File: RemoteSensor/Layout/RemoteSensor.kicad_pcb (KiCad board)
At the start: 2 copper layers, 50.8 x 50.8 mm, 47 parts, among them J1 PRG_HEADER, J2 LCD_HEADER, J3 USB_B_Micro, J4 BATT_CONN, Q1 2N7002, Q2 2N7002, Q3 2N7002, SW1 BTN_RST, SW2 BTN_LOAD, SW3 SW_DPDT_x2, U1 ESP-12F, U2 74LVC2G02, U3 LM50CIM3, U4 MCP73831-2-OT, U5 LM3670MF, U6 BD48ExxG, U7 BD48ExxG

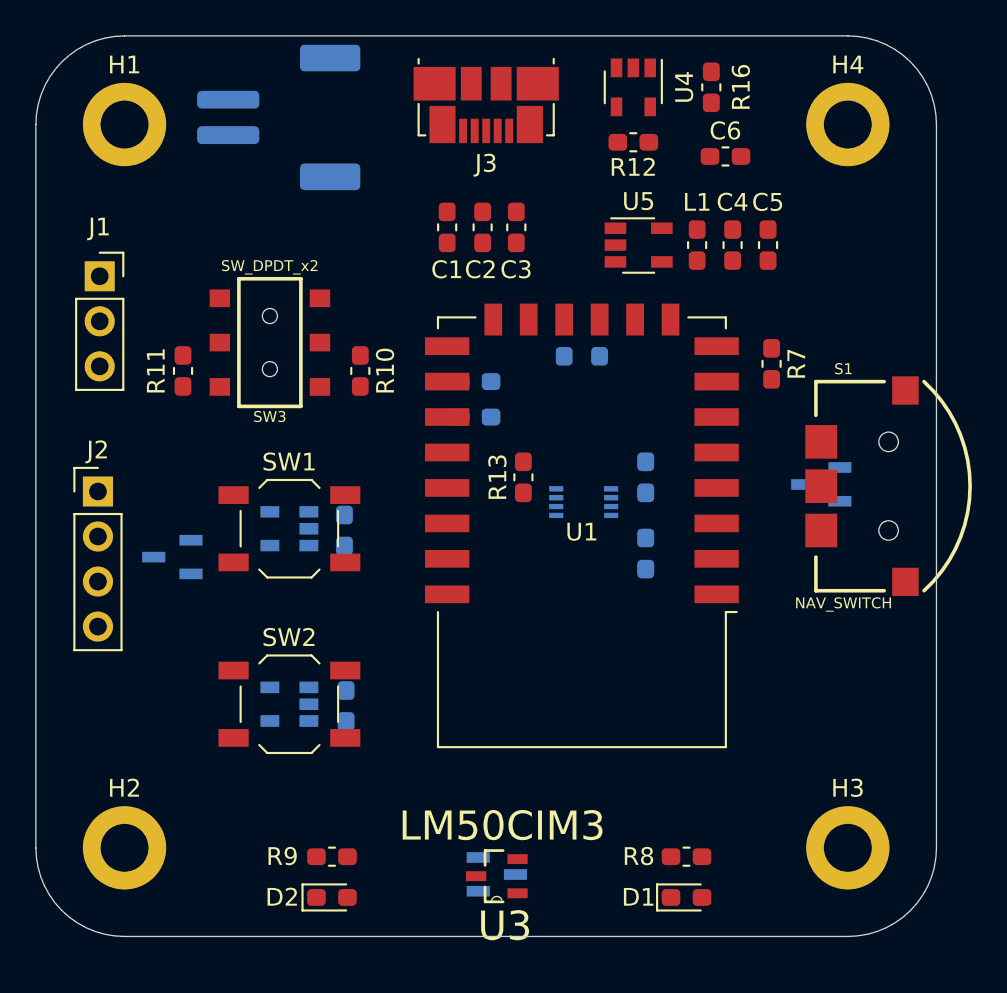
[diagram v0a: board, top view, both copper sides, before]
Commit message: Autotrace
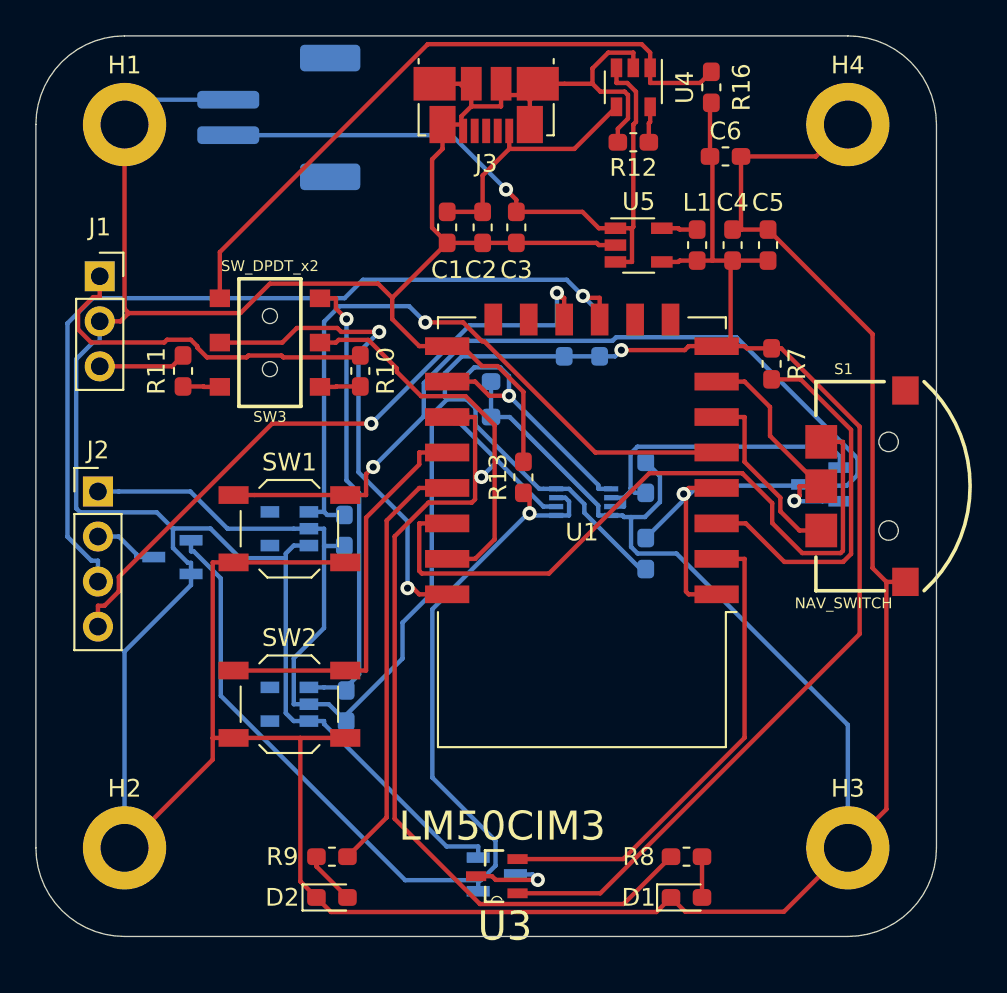
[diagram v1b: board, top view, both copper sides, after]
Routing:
- net GND: track 0.00 -> 335.7 mm
- net 3.3V: track 0.00 -> 149.5 mm, vias 0 -> 1
- net /RST: track 0.00 -> 67.6 mm, vias 0 -> 2
- net /WAKE_STS: track 0.00 -> 59.2 mm, vias 0 -> 1
- net /HB_PIN: track 0.00 -> 55.6 mm, vias 0 -> 1
- net /SCL: track 0.00 -> 50.2 mm, vias 0 -> 1
- net /UP_PIN: track 0.00 -> 40.5 mm
- net /BATT_STS: track 0.00 -> 38.7 mm, vias 0 -> 1
- net V_BATT: track 0.00 -> 38.1 mm, vias 0 -> 1
- net /SDA: track 0.00 -> 38.1 mm, vias 0 -> 2
- net /CHARGE_STS: track 0.00 -> 37.4 mm
- net /RADIO_TX: track 0.00 -> 27.9 mm, vias 0 -> 2
- net /TEMP_PIN: track 0.00 -> 27.3 mm
- net /CHARGER_STS: track 0.00 -> 26.0 mm, vias 0 -> 1
- net /BATT_PIN: track 0.00 -> 24.1 mm
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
